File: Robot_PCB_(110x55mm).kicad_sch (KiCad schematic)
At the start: 21 parts, among them U1 L293, U2 SW_DPDT_XLX, U3 AMS1117-5.0, U5 MFRC522 37.5x25mm

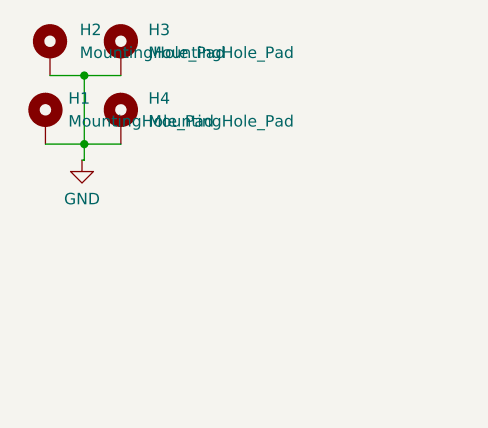
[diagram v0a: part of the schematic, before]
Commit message: Update
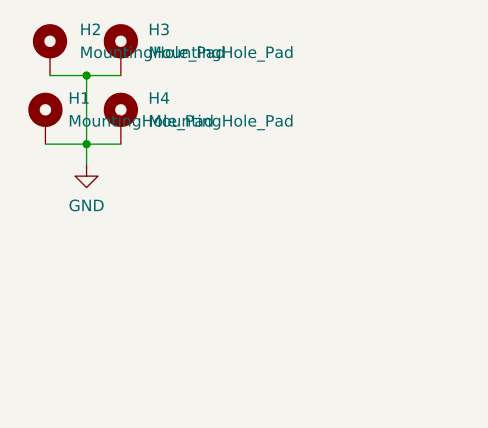
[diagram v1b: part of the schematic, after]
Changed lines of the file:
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@@
     (company "GERE")
   )
-  (junction (at 20.574 27.432) (diameter 0) (color 0 0 0 0)
-  )
   (junction (at 51.308 98.298) (diameter 0) (color 0 0 0 0)
   )
@@
   (junction (at 201.295 45.212) (diameter 0) (color 0 0 0 0)
   )
-  (junction (at 20.574 19.812) (diameter 0) (color 0 0 0 0)
+  (junction (at 20.828 19.812) (diameter 0) (color 0 0 0 0)
   )
   (junction (at 51.308 105.918) (diameter 0) (color 0 0 0 0)
@@
   (junction (at 207.645 32.512) (diameter 0) (color 0 0 0 0)
   )
+  (junction (at 20.828 27.432) (diameter 0) (color 0 0 0 0)
+  )
   (junction (at 181.61 45.847) (diameter 0) (color 0 0 0 0)
   )
@@
     (stroke (width 0) (type default))
   )
+  (wire (pts (xy 20.828 19.812) (xy 24.638 19.812))
+    (stroke (width 0) (type default))
+  )
   (wire (pts (xy 122.555 89.535) (xy 125.73 89.535))
     (stroke (width 0) (type default))
@@
     (stroke (width 0) (type default))
   )
+  (wire (pts (xy 20.828 29.718) (xy 20.828 27.432))
+    (stroke (width 0) (type default))
+  )
   (wire (pts (xy 104.14 41.91) (xy 110.49 41.91))
     (stroke (width 0) (type default))
@@
     (stroke (width 0) (type default))
   )
-  (wire (pts (xy 20.574 19.812) (xy 24.638 19.812))
-    (stroke (width 0) (type default))
-  )
   (wire (pts (xy 144.526 36.322) (xy 144.526 37.592))
     (stroke (width 0) (type default))
@@
     (stroke (width 0) (type default))
   )
-  (wire (pts (xy 20.574 27.432) (xy 20.574 29.21))
-    (stroke (width 0) (type default))
-  )
   (wire (pts (xy 44.704 81.28) (xy 44.704 81.534))
     (stroke (width 0) (type default))
@@
     (stroke (width 0) (type default))
   )
-  (wire (pts (xy 20.574 29.21) (xy 20.32 29.21))
+  (wire (pts (xy 20.828 27.432) (xy 20.828 19.812))
     (stroke (width 0) (type default))
   )
@@
     (stroke (width 0) (type default))
   )
-  (wire (pts (xy 16.764 19.812) (xy 20.574 19.812))
-    (stroke (width 0) (type default))
-  )
   (wire (pts (xy 122.555 109.855) (xy 125.73 109.855))
     (stroke (width 0) (type default))
@@
     (stroke (width 0) (type default))
   )
+  (wire (pts (xy 20.828 27.432) (xy 24.638 27.432))
+    (stroke (width 0) (type default))
+  )
   (wire (pts (xy 93.218 93.98) (xy 90.678 93.98))
     (stroke (width 0) (type default))
@@
     (stroke (width 0) (type default))
   )
-  (wire (pts (xy 20.574 27.432) (xy 24.638 27.432))
-    (stroke (width 0) (type default))
-  )
   (wire (pts (xy 181.61 32.512) (xy 181.61 38.227))
     (stroke (width 0) (type default))
@@
     (stroke (width 0) (type default))
   )
-  (wire (pts (xy 20.574 19.812) (xy 20.574 27.432))
-    (stroke (width 0) (type default))
-  )
   (wire (pts (xy 236.093 141.478) (xy 236.093 142.24))
     (stroke (width 0) (type default))
@@
     (stroke (width 0) (type default))
   )
-  (wire (pts (xy 16.256 27.432) (xy 20.574 27.432))
+  (wire (pts (xy 16.764 19.812) (xy 20.828 19.812))
     (stroke (width 0) (type default))
   )
@@
   )
   (wire (pts (xy 201.295 45.212) (xy 201.295 45.847))
+    (stroke (width 0) (type default))
+  )
+  (wire (pts (xy 16.256 27.432) (xy 20.828 27.432))
     (stroke (width 0) (type default))
   )
@@
         (path "/5740c1d8-40a5-48a4-b0ff-1fed8540b5f6"
           (reference "U3") (unit 1)
+        )
+      )
+    )
+  )
+  (symbol (lib_id "power:GND") (at 20.828 29.718 0) (unit 1)
+    (in_bom yes) (on_board yes) (dnp no) (fields_autoplaced)
+    (property "Reference" "#PWR026" (at 20.828 36.068 0)
+      (effects (font (size 1.27 1.27)) hide)
+    )
+    (property "Value" "GND" (at 20.828 34.29 0)
+      (effects (font (size 1.27 1.27)))
+    )
+    (property "Footprint" "" (at 20.828 29.718 0)
+      (effects (font (size 1.27 1.27)) hide)
+    )
+    (property "Datasheet" "" (at 20.828 29.718 0)
+      (effects (font (size 1.27 1.27)) hide)
+    )
+    (pin "1")
+    (instances
+      (project "Robot_PCB_(110x55mm)"
+        (path "/5740c1d8-40a5-48a4-b0ff-1fed8540b5f6"
+          (reference "#PWR026") (unit 1)
         )
       )
@@
         )
       )
-    )
-  )
-  (symbol (lib_id "power:GND") (at 20.32 29.21 0) (unit 1)
-    (in_bom yes) (on_board yes) (dnp no) (fields_autoplaced)
-    (property "Reference" "#PWR026" (at 20.32 35.56 0)
-      (effects (font (size 1.27 1.27)) hide)
-    )
-    (property "Value" "GND" (at 20.32 33.528 0)
-      (effects (font (size 1.27 1.27)))
-    )
-    (property "Footprint" "" (at 20.32 29.21 0)
-      (effects (font (size 1.27 1.27)) hide)
-    )
-    (property "Datasheet" "" (at 20.32 29.21 0)
-      (effects (font (size 1.27 1.27)) hide)
-    )
-    (pin "1")
-    (instances
-      (project "Robot_PCB_(110x55mm)"
-        (path "/5740c1d8-40a5-48a4-b0ff-1fed8540b5f6"
-          (reference "#PWR026") (unit 1)
-        )
-      )
